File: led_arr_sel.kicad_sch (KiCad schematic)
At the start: 4 parts

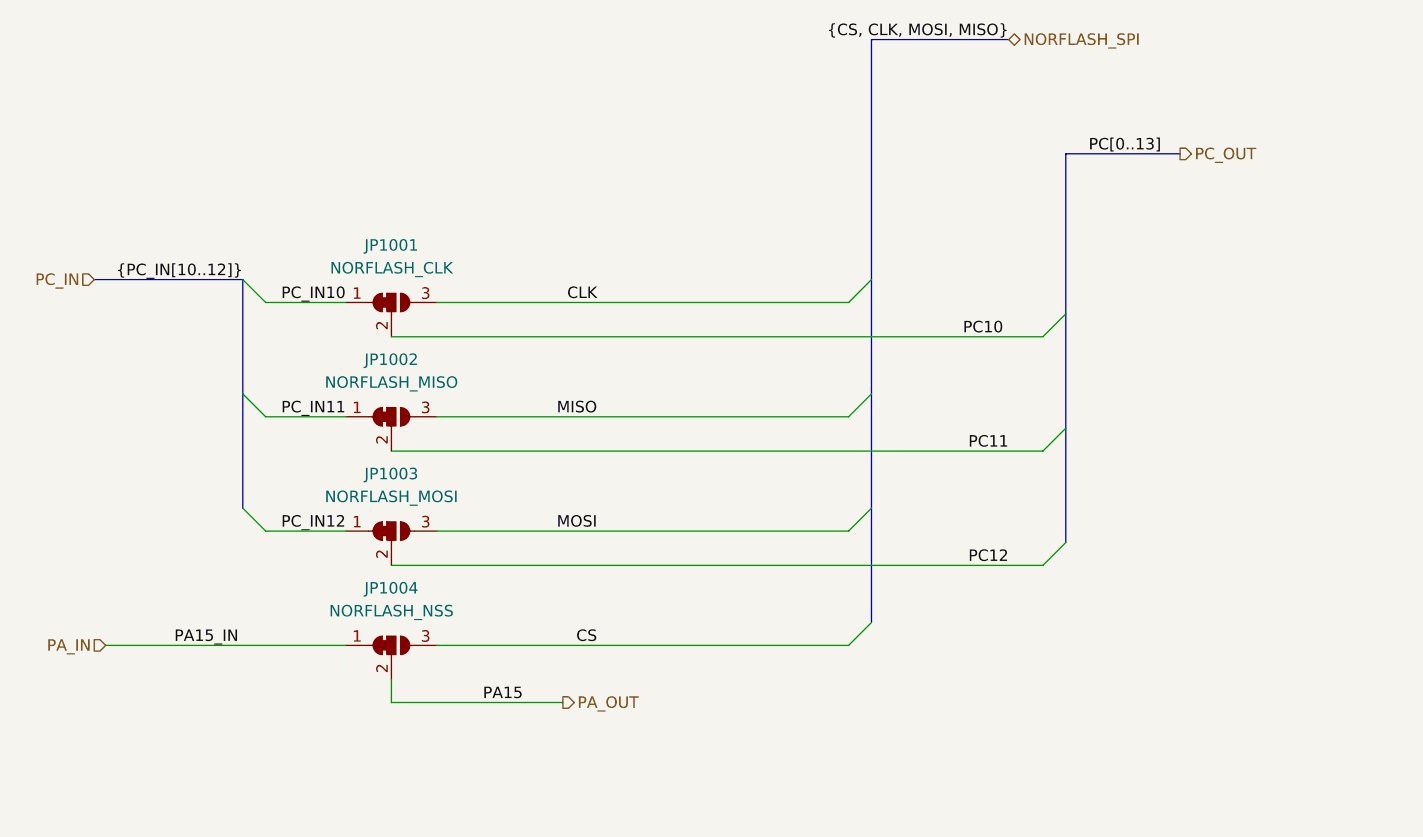
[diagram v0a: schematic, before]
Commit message: fixed like a bunch of things, power and new xcvr and lights and other goodies, also started layout
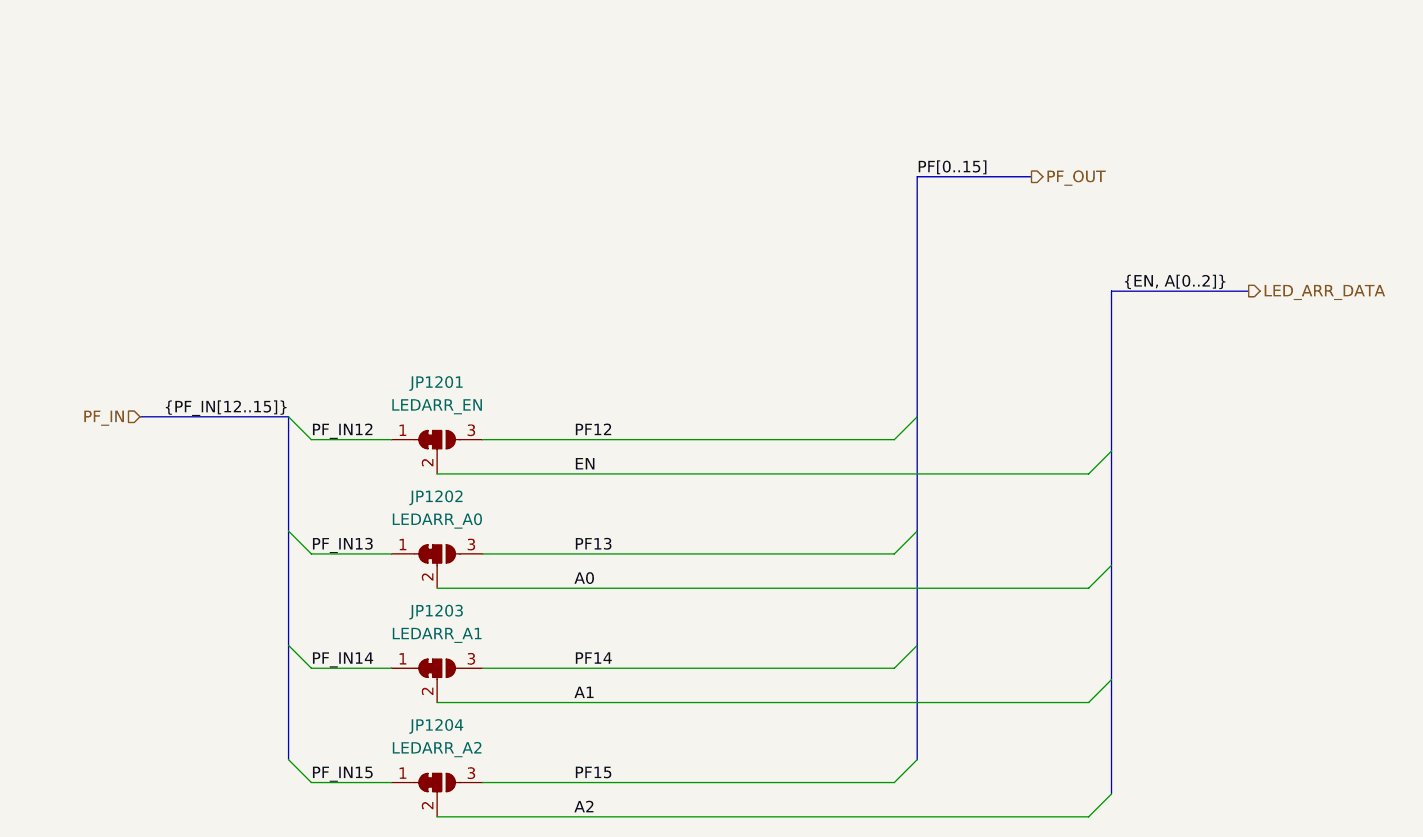
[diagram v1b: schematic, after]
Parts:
- removed JP1001: NORFLASH_CLK, Jumper:SolderJumper-3_P1.3mm_Bridged2Bar12_Pad1.0x1.5mm_NumberLabels, symbol Jumper:SolderJumper_3_Bridged12
- removed JP1002: NORFLASH_MISO, Jumper:SolderJumper-3_P1.3mm_Bridged2Bar12_Pad1.0x1.5mm_NumberLabels, symbol Jumper:SolderJumper_3_Bridged12
- removed JP1003: NORFLASH_MOSI, Jumper:SolderJumper-3_P1.3mm_Bridged2Bar12_Pad1.0x1.5mm_NumberLabels, symbol Jumper:SolderJumper_3_Bridged12
- removed JP1004: NORFLASH_NSS, Jumper:SolderJumper-3_P1.3mm_Bridged2Bar12_Pad1.0x1.5mm_NumberLabels, symbol Jumper:SolderJumper_3_Bridged12
- added JP1201: LEDARR_EN, Jumper:SolderJumper-3_P1.3mm_Bridged2Bar12_Pad1.0x1.5mm_NumberLabels, symbol Jumper:SolderJumper_3_Bridged12
- added JP1202: LEDARR_A0, Jumper:SolderJumper-3_P1.3mm_Bridged2Bar12_Pad1.0x1.5mm_NumberLabels, symbol Jumper:SolderJumper_3_Bridged12
- added JP1203: LEDARR_A1, Jumper:SolderJumper-3_P1.3mm_Bridged2Bar12_Pad1.0x1.5mm_NumberLabels, symbol Jumper:SolderJumper_3_Bridged12
- added JP1204: LEDARR_A2, Jumper:SolderJumper-3_P1.3mm_Bridged2Bar12_Pad1.0x1.5mm_NumberLabels, symbol Jumper:SolderJumper_3_Bridged12
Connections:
- new net A0: JP1202.2 (C)
- new net A1: JP1203.2 (C)
- new net A2: JP1204.2 (C)
- new net EN: JP1201.2 (C)
- new net PF12: JP1201.3 (B)
- new net PF13: JP1202.3 (B)
- new net PF14: JP1203.3 (B)
- new net PF15: JP1204.3 (B)
- new net PF_IN12: JP1201.1 (A)
- new net PF_IN13: JP1202.1 (A)
- new net PF_IN14: JP1203.1 (A)
- new net PF_IN15: JP1204.1 (A)
